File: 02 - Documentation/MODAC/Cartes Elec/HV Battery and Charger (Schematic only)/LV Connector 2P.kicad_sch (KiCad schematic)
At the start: 0 parts

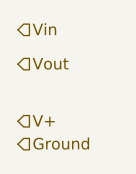
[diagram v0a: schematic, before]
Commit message: Update schematique chargeur
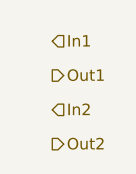
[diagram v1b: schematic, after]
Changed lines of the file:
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@@
 	(generator_version "8.0")
 	(paper "A4")
-	(hierarchical_label "Ground"
-		(shape input)
-		(at 125.73 86.36 0)
+	(hierarchical_label "Out1"
+		(shape output)
+		(at 129.54 78.74 0)
 		(fields_autoplaced yes)
 		(effects
@@
 		)
 	)
-	(hierarchical_label "Vout"
-		(shape input)
-		(at 125.73 77.47 0)
+	(hierarchical_label "Out2"
+		(shape output)
+		(at 129.54 86.36 0)
 		(fields_autoplaced yes)
 		(effects
@@
 		)
 	)
-	(hierarchical_label "V+"
+	(hierarchical_label "In2"
 		(shape input)
-		(at 125.73 83.82 0)
+		(at 129.54 82.55 0)
 		(fields_autoplaced yes)
 		(effects
@@
 		)
 	)
-	(hierarchical_label "Vin"
+	(hierarchical_label "In1"
 		(shape input)
-		(at 125.73 73.66 0)
+		(at 129.54 74.93 0)
 		(fields_autoplaced yes)
 		(effects
